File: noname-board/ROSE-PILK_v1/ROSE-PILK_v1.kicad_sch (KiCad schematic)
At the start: 4 parts, among them J2 Conn_01x03, SW1 SW_Push, SW2 SW_Push

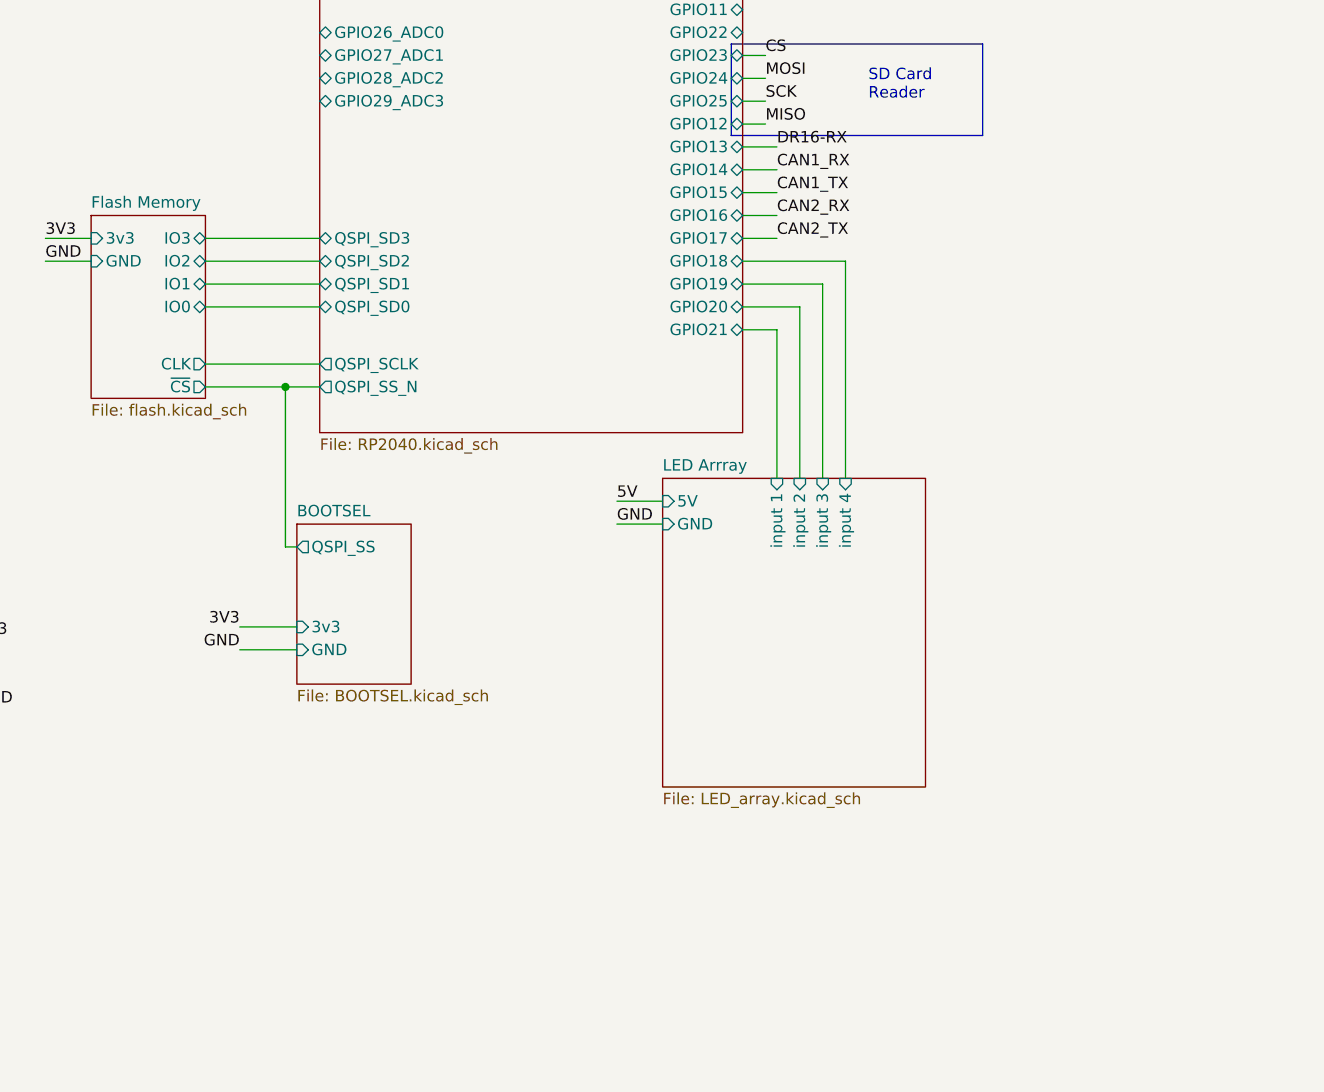
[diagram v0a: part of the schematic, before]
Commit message: v1 functionality finished
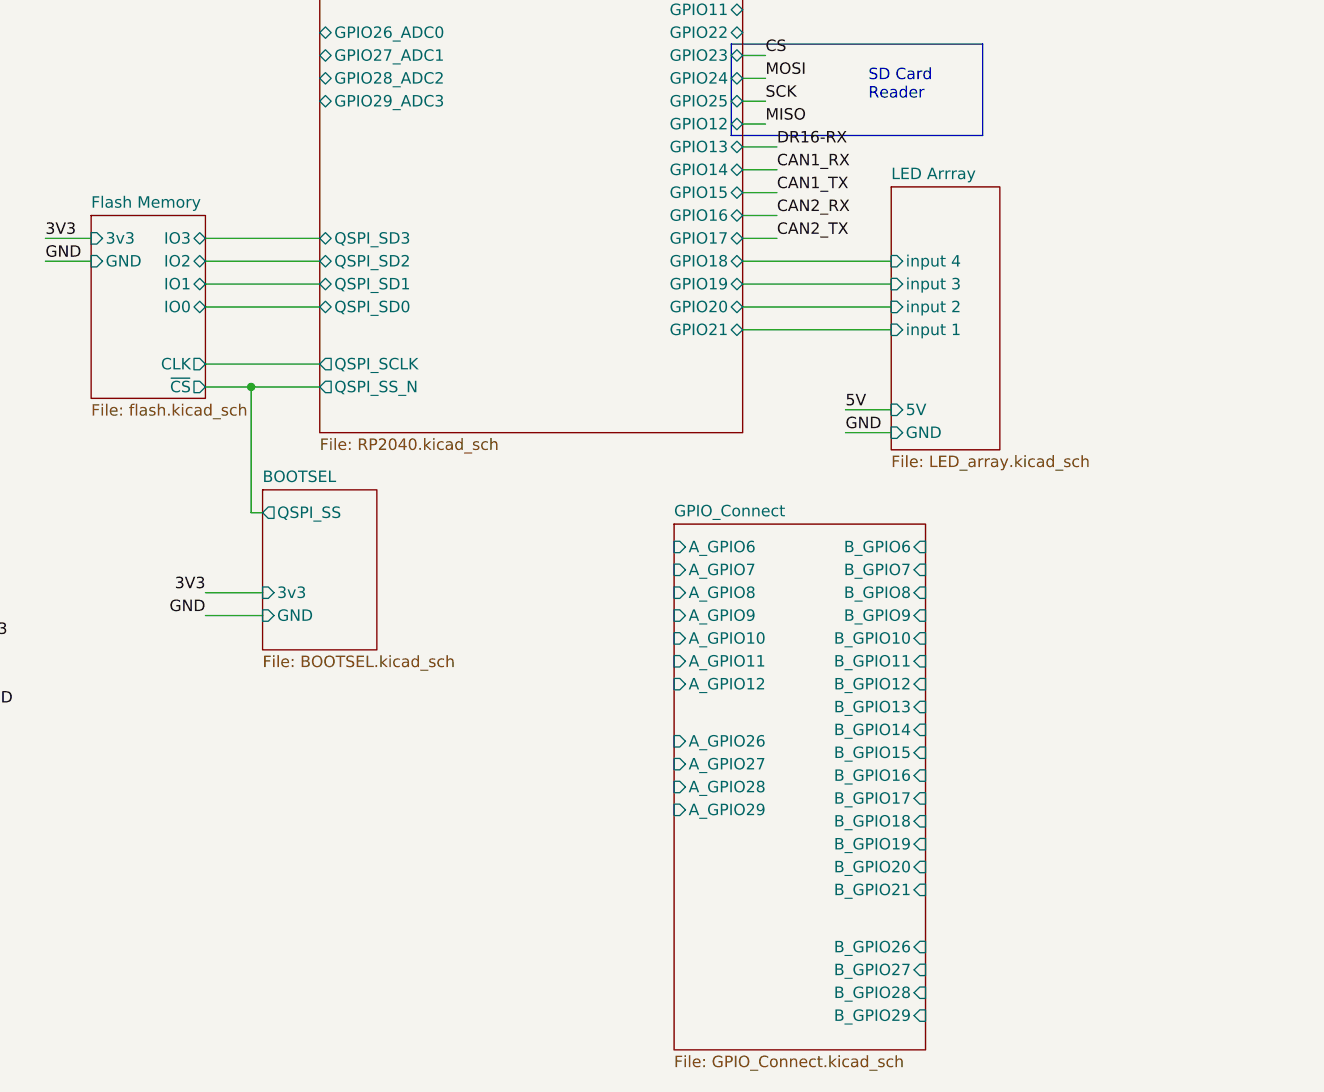
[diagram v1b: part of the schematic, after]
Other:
- added sheet GPIO_Connect (GPIO_Connect.kicad_sch)
